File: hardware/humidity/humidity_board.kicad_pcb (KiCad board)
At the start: 2 copper layers, 100 x 20 mm, 25 parts, among them IC1 ATMEGA88-A, J1 RJ45, P1 ISP, P2 UART, SW1 SW_RESET, U1 ST485, U2 HYT271, m3_loch VAL**

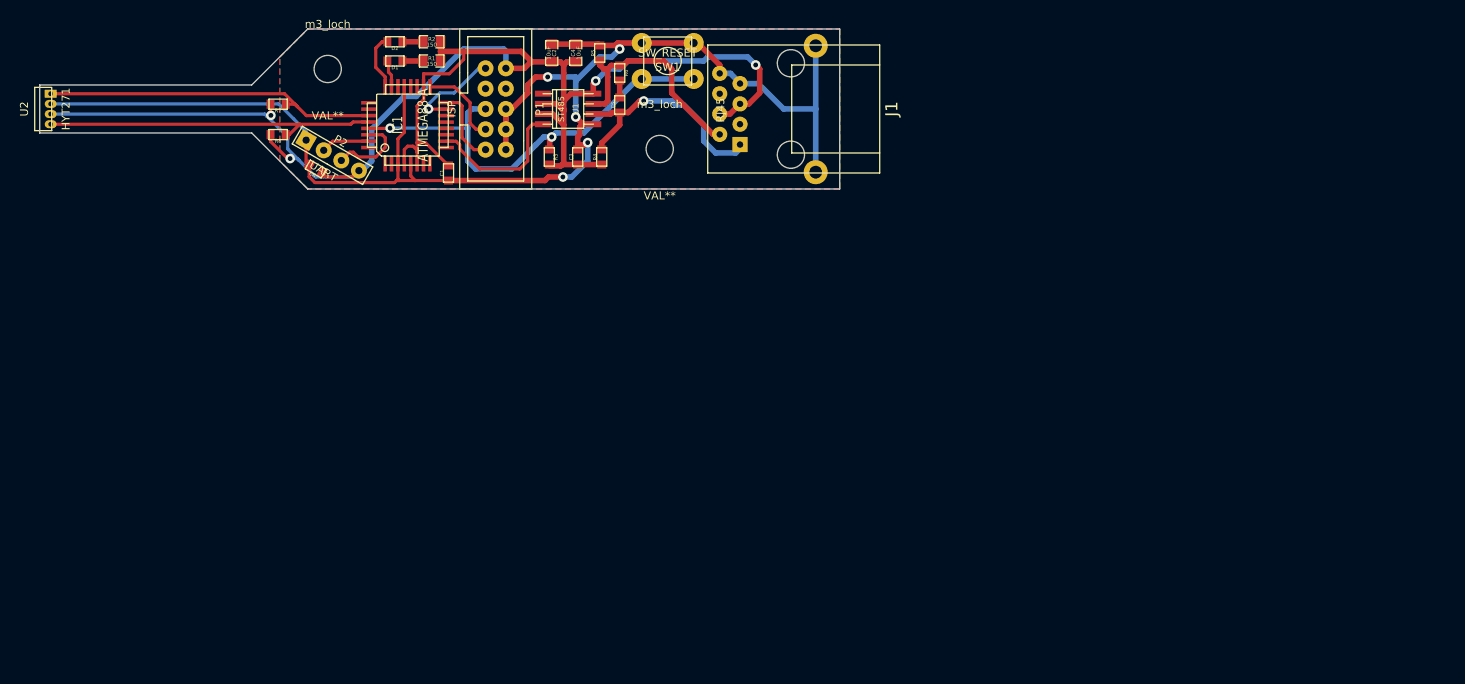
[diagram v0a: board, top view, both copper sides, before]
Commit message: for put all together
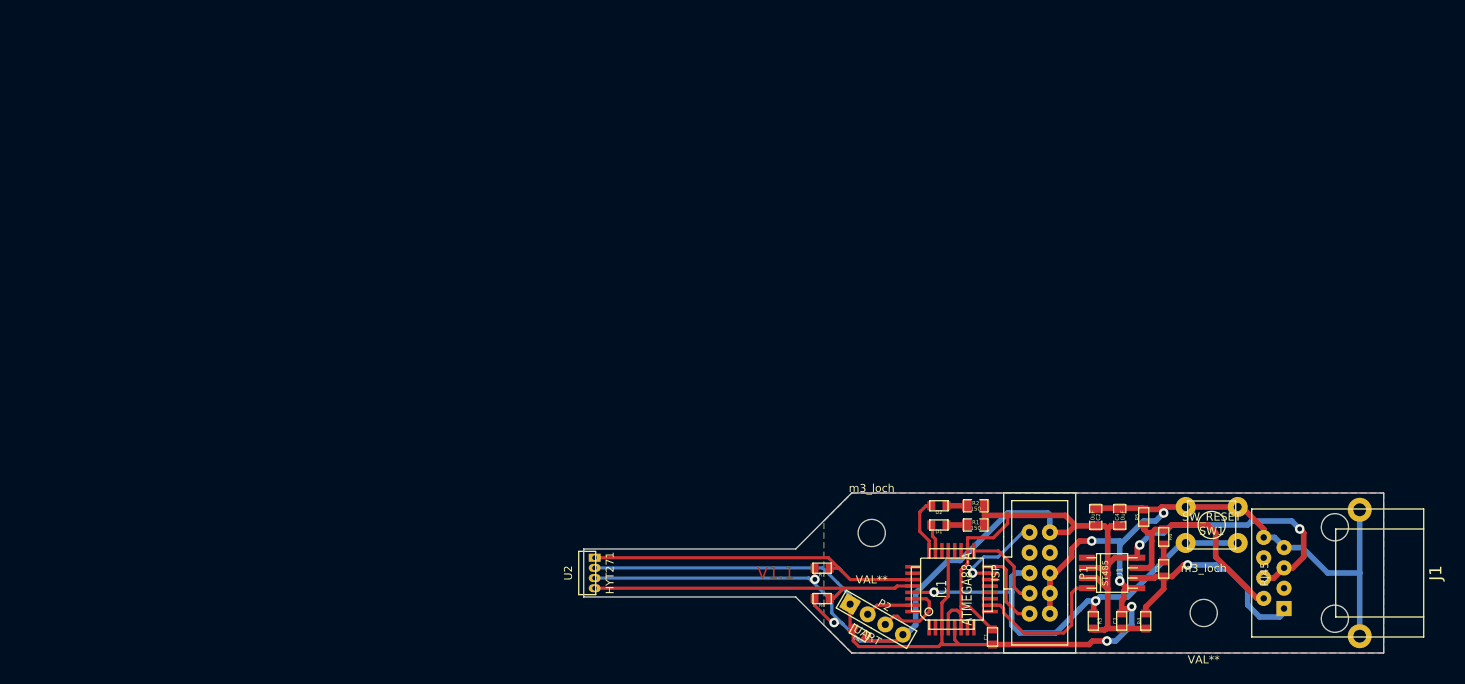
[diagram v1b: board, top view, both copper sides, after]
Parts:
- moved P2 89.4 mm to (204.6, 159.8)
- moved C1 89.4 mm to (219.1, 162.0)
- moved C2 89.4 mm to (232.0, 147.0)
- moved C3 89.4 mm to (235.2, 160.0)
- moved C4 89.4 mm to (235.0, 147.0)
- moved C5 89.4 mm to (240.5, 153.5)
- moved C6 89.4 mm to (202.5, 161.5)
- moved D1 89.4 mm to (212.4, 148.0)
- moved D2 89.4 mm to (212.4, 145.6)
- moved IC1 89.4 mm to (214.0, 156.0)
- moved J1 89.4 mm to (253.0, 154.0)
- moved P1 89.4 mm to (225.0, 154.0)
- moved R1 89.4 mm to (217.0, 148.0)
- moved R2 89.4 mm to (217.0, 145.6)
- moved R3 89.4 mm to (231.7, 160.0)
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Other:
- board text added: "V1.1"
